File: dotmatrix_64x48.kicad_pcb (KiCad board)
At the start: 2 copper layers, 207 x 120 mm, 372 parts, among them J7 Conn_01x04_Female, P1 CONN_01X06, P2 CONN_01X06, P3 CONN_01X08, P4 CONN_01X08, Q1 Q_NPN_BCE RN5006, Q10 AO3401, Q11 AO3401, Q12 AO3401, Q13 AO3401, Q14 AO3401, Q15 AO3401, Q16 AO3401, Q17 AO3401, Q18 AO3401, Q19 AO3401, Q2 Q_NPN_BEC, Q20 AO3401, Q21 AO3401, Q22 AO3401, Q23 AO3401, Q24 AO3401, Q25 AO3401, Q26 AO3401, Q27 AO3401, Q28 AO3401, Q29 AO3401, Q3 NJL7302L-F3, Q30 Q_NPN_BEC, Q4 Q_NPN_BEC, Q5 AO3401, Q6 AO3401, Q7 AO3401, Q8 AO3401, Q9 AO3401, SW1 SW_PUSH_SMALL_H, SW2 SW_PUSH_SMALL_H, SW3 SW_PUSH_SMALL_H, SW4 SW_PUSH_SMALL_H, SW5 SW_PUSH_SMALL_H, SW6 SW_PUSH_SMALL_H, SW7 SW_PUSH_SMALL_H, SW8 SW_PUSH_SMALL_H, T1 COMMON_MODE_CHOKE, U1 74VHC541, U10 LED1642GW, U11 74HC595, U12 AE-BME280, U13 74HC595, U14 MAX98357, U15 74HC595, U16 ESP32-WROOM, U17 OSRB38C9AA, U18 BME280, U19 TPS54428DDA, U2 TPS54202, U20 CP2102N-A01-GQFN28, U21 CM1293A-04SO, U22 CM1293A-04SO, U23 CM1293A-04SO, U24 CM1293A-04SO, U25 CM1293A-04SO, U3 LED1642GW, U4 LED1642GW, U5 LED1642GW, U6 LED1642GW, U7 LED1642GW, U8 LED1642GW, U9 LED1642GW

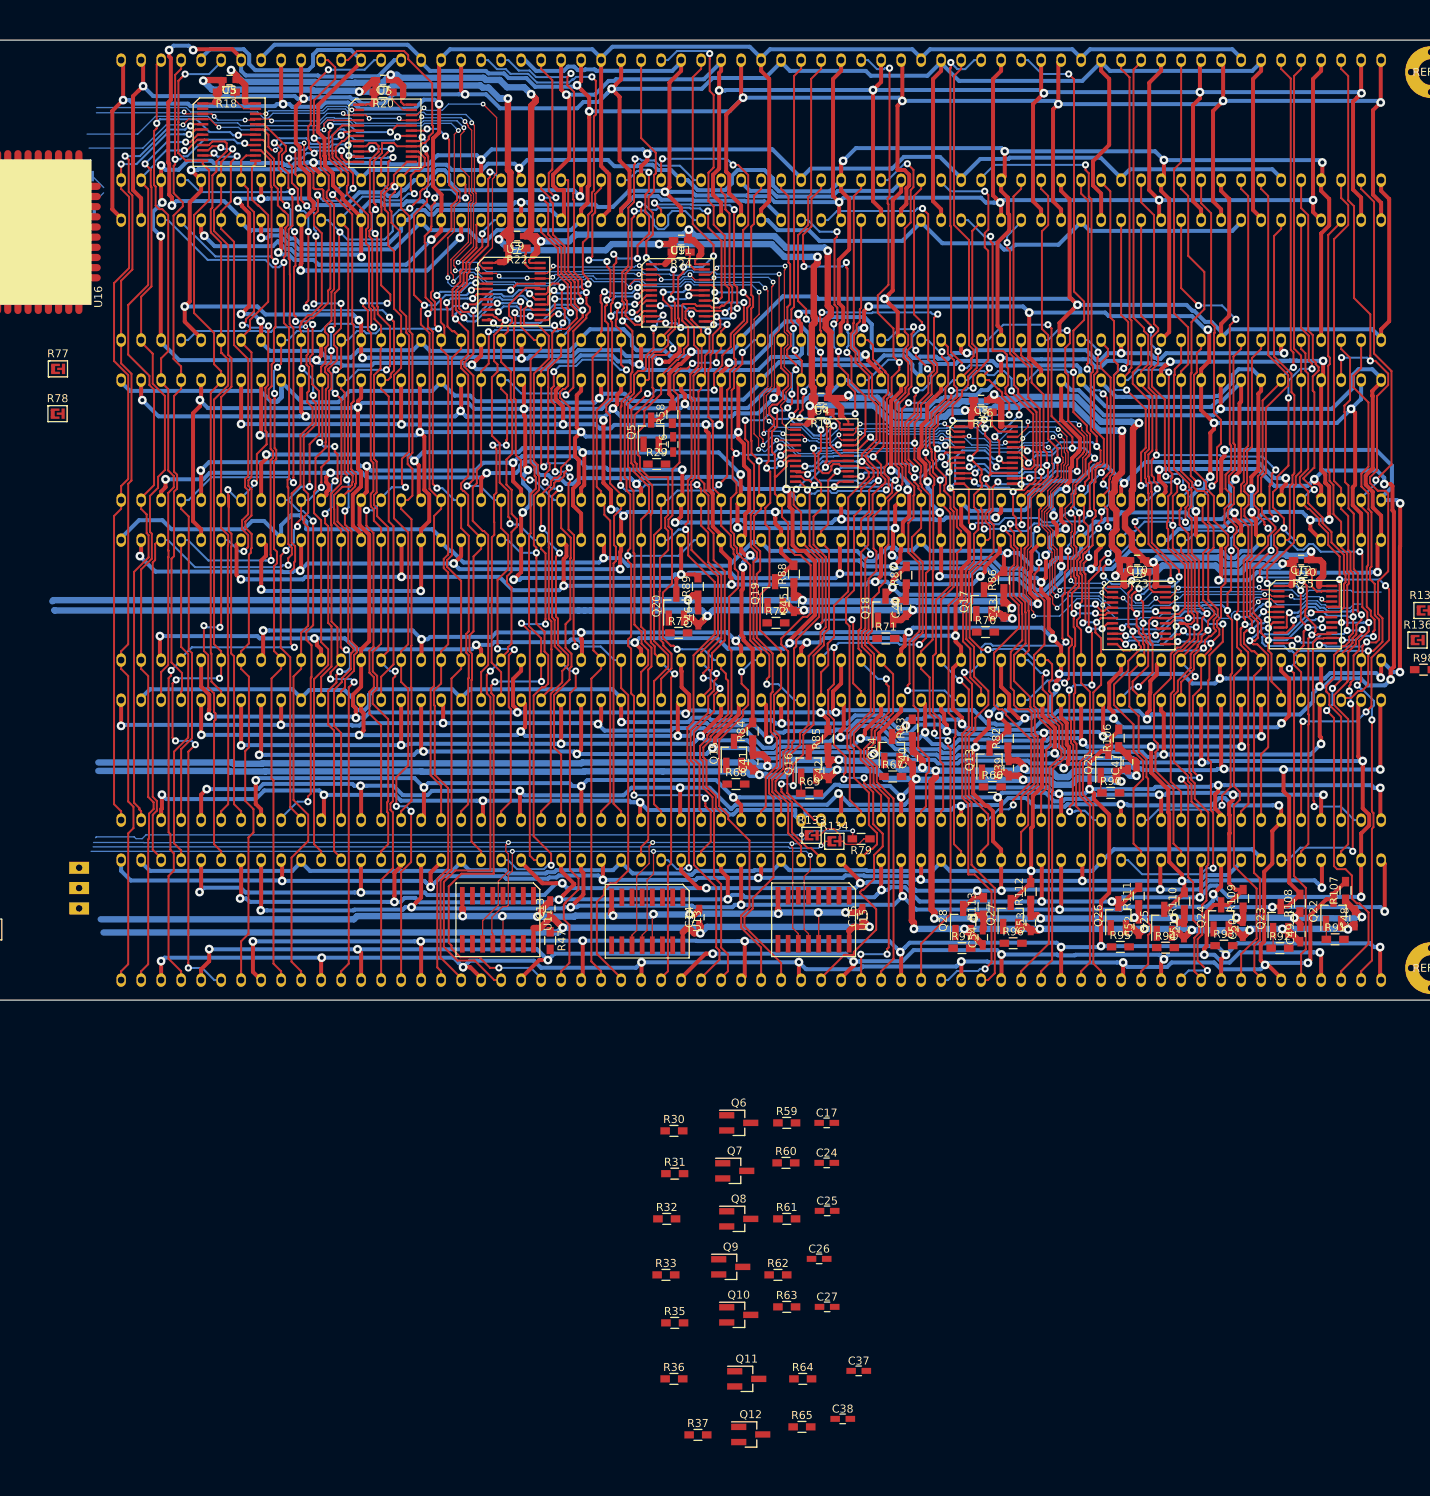
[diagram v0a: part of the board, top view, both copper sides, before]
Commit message: Getting very mojai
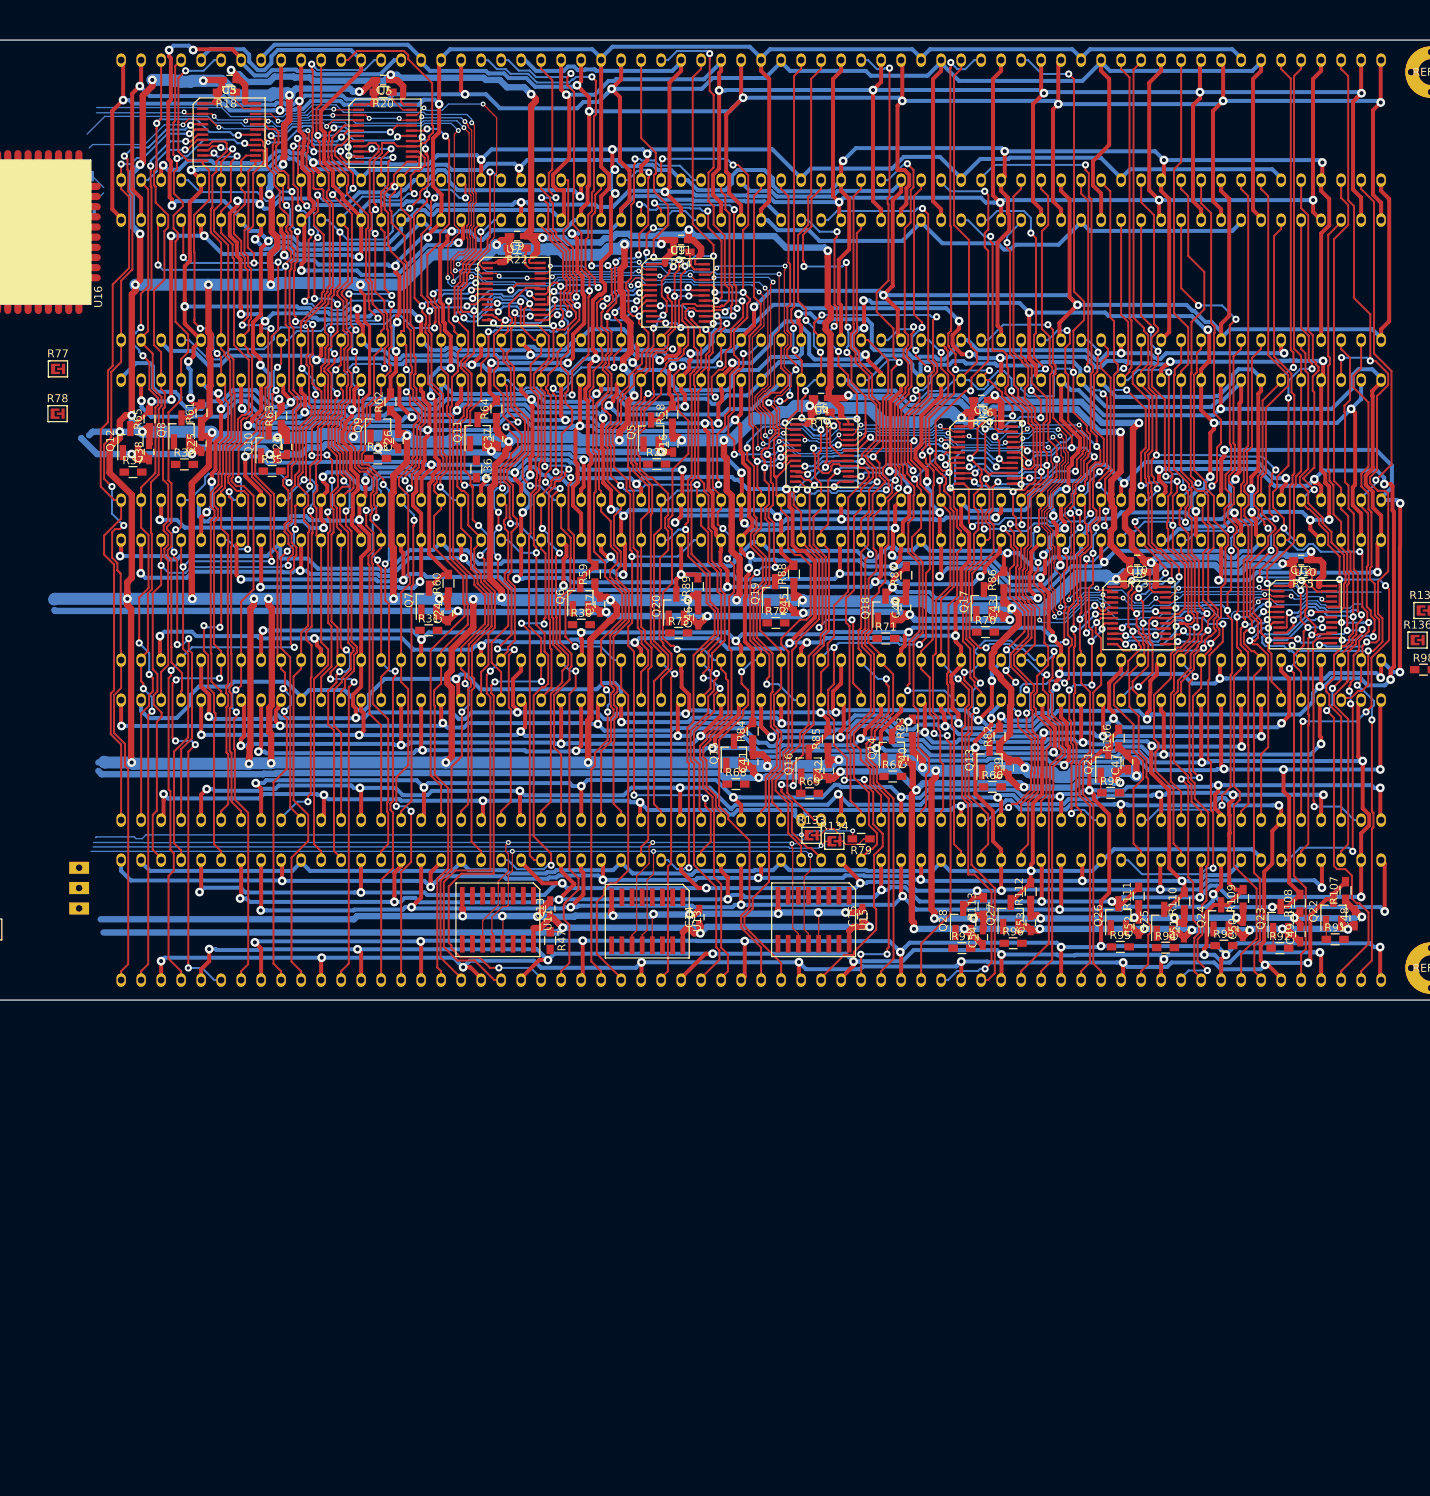
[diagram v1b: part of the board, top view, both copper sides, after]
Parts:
- moved R65 150.1 mm to (121.8, 63.4), turned to 90 degrees
- moved C38 148.7 mm to (121.7, 67.5), turned to 90 degrees
- moved Q12 146.4 mm to (119.4, 66.1), turned to 90 degrees
- moved R37 139.5 mm to (119.7, 70.0)
- moved R63 128.1 mm to (138.3, 63.0), turned to 90 degrees
- moved R64 127.1 mm to (165.2, 62.1), turned to 90 degrees
- moved C27 126.9 mm to (139.0, 66.8), turned to 90 degrees
- moved C37 124.9 mm to (165.4, 65.9), turned to 90 degrees
- moved R61 124.5 mm to (128.3, 62.6), turned to 90 degrees
- moved C25 123.8 mm to (128.3, 66.5), turned to 90 degrees
- moved Q10 123.7 mm to (136.7, 66.5), turned to 90 degrees
- moved Q11 123.1 mm to (162.8, 65.0), turned to 90 degrees
- moved Q8 120.7 mm to (125.8, 64.7), turned to 90 degrees
- moved R62 119.4 mm to (151.9, 61.2), turned to 90 degrees
- moved R35 117.8 mm to (137.1, 69.9)
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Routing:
- net GND: track 829.2 -> 1334.7 mm, vias 38 -> 75
- net LEDVDD: track 531.7 -> 635.3 mm, vias 20 -> 28
- net r2: track 317.5 -> 370.1 mm, vias 8 -> 11
- net r6: track 336.3 -> 380.4 mm, vias 6 -> 9
- net r1: track 354.3 -> 397.1 mm, vias 13 -> 14
- net r15: track 357.0 -> 389.9 mm, vias 15 -> 21
- net r7: track 330.9 -> 361.9 mm, vias 8 -> 11
- net r5: track 336.4 -> 363.9 mm, vias 9 -> 12
- net r4: track 331.7 -> 351.7 mm, vias 5 -> 8
- net r3: track 344.3 -> 359.5 mm, vias 11 -> 12
- net co18: track 94.7 -> 104.9 mm, vias 3 -> 8
- net r12: track 354.1 -> 361.9 mm, vias 5 -> 7
- net r22: track 341.7 -> 349.4 mm, vias 7 -> 8
- net r14: track 363.2 -> 369.7 mm, vias 19 -> 18
- net ce52: track 110.5 -> 116.9 mm, vias 8 -> 10
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
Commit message: Almost all components has placed.
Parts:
- removed C36: 1u, Capacitors_SMD:C_0603_HandSoldering
- removed C63: 0.1u, Capacitors_SMD:C_0603_HandSoldering
- removed P3, P4: CONN_01X08, Pin_Headers:Pin_Header_Straight_1x08_Pitch2.54mm
- removed R1: 1k, Resistors_SMD:R_0603_HandSoldering
- removed U18: BME280, components:BME280-handsoldering
- removed W1, W10, W12, W13, W14, W15, W16, W17, W18, W19, W2, W3, W4, W7: TEST_1P, Measurement_Points:Measurement_Point_Round-SMD-Pad_Small
- added J1: Conn_02x04_Odd_Even, Pin_Headers:Pin_Header_Angled_2x04_Pitch2.54mm, F.Cu at (107.0, 22.2)
- added J2: Conn_02x04_Odd_Even, Pin_Headers:Pin_Header_Angled_2x04_Pitch2.54mm, F.Cu at (114.6, 123.0)
- added REF**: SPK_DAEX25FHE-4_adhesive_circle, components:SPK_DAEX25FHE-4_adhesive_circle, F.Cu at (185.7, 75.9)
- C2, C21, C22, C23, C3, C4, C62, C64, C65, C66, C72, D12, D14, D7, F1, L3, L6, LED49, LED50, LED51, Q1, Q3, R100, R11, R118, R119, R12, R120, R121, R125, R126, R127, R128, R13, R130, R131, R132, R14, R15, R2, R27, R34, R4, R41, R42, R46, R49, R5, R51, R54, R55, R57, R6, R7, R74, R75, R76, R8, U1, U12, U16: moved to B.Cu
- C28, C33: value 10u -> 10u 16V
- C75, C76: value 1u -> 1u 16V
- L1: value 2.2uH -> 10uH; footprint components:Choke_SMD_12x12mm_10.4x10.4mm_compat_h4.5mm_handsoldering -> components:Choke_SMD_7.3x7.3_H3.5_handsoldering
- L2: footprint components:Choke_SMD_12x12mm_10.4x10.4mm_compat_h4.5mm_handsoldering -> components:Choke_SMD_7.3x7.3_H3.5_handsoldering
- LS1: footprint components:SPK_35mm_20mm_RECTANGLE_MOUNT -> Wire_Connections_Bridges:WireConnection_1.50mmDrill
- R80, R81: moved to F.Cu
- moved U25 694.8 mm to (86.2, 46.5)
- moved R34 659.0 mm to (103.2, 18.6), turned to 90 degrees
- moved R118 656.7 mm to (104.5, 20.8), turned to 90 degrees
- moved R127 650.6 mm to (107.2, 17.2)
- moved R121 649.6 mm to (106.8, 28.1), turned to 270 degrees
- moved R119 649.6 mm to (103.0, 28.1), turned to 90 degrees
- moved R120 647.9 mm to (104.2, 28.1), turned to 90 degrees
- moved R128 647.6 mm to (98.0, 53.4), turned to 90 degrees
- moved R132 647.4 mm to (108.8, 53.4), turned to 90 degrees
- moved R130 644.4 mm to (105.8, 53.4), turned to 90 degrees
- moved U22 644.1 mm to (94.7, 104.9), turned to 90 degrees
- moved R126 642.5 mm to (111.1, 17.2)
- moved R122 640.6 mm to (117.1, 21.0), turned to 90 degrees
- moved U21 640.1 mm to (103.0, 132.0), turned to 90 degrees
- moved R125 639.4 mm to (114.9, 17.2), turned to 180 degrees
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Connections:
- net DC_IN renamed DC_IN_P
- net Net-(C72-Pad2) renamed /power/DC_IN_N
- net Net-(CONN3-Pad2) renamed /IR_Sensor/IRLED_K
- net Net-(LS1-Pad1) renamed /IR_Sensor/SPK_P
- net Net-(LS1-Pad2) renamed /IR_Sensor/SPK_N
- C1 pad 1: Net-(C1-Pad1) -> /IR_Sensor/FILT_VDD
- C32 pad 1: Net-(C1-Pad1) -> /IR_Sensor/FILT_VDD
- C4 pad 1: VCC -> LEDVDD
- C67 pad 1: GND -> /USB_UART/USB3V3
- C70 pad 1: GND -> /USB_UART/USB3V3
- C73 pad 1: GND -> /USB_UART/USB3V3
- J7 pad 4: ESPVDD -> LEDLOGICVDD
- L6 pad 1: VCC -> LEDVDD
- P2 pad 1: GND -> /USB_UART/USB3V3
- R10 pad 2: ESPVDD -> LEDLOGICVDD
- R117 pad 2: GND -> /USB_UART/USB3V3
- R123 pad 1: Net-(C1-Pad1) -> /IR_Sensor/FILT_VDD
- R124 pad 1: Net-(C1-Pad1) -> /IR_Sensor/FILT_VDD
- R16 pad 2: VCC -> LEDVDD
- R17 pad 2: VCC -> LEDVDD
- R26 pad 2: VCC -> LEDVDD
- R28 pad 1: ESPVDD -> LEDLOGICVDD
- R45 pad 2: ESPVDD -> /IR_Sensor/FILT_VDD
- R9 pad 2: ESPVDD -> LEDLOGICVDD
- U12 pad 1: ESPVDD -> LEDLOGICVDD
- U17 pad 3: Net-(C1-Pad1) -> /IR_Sensor/FILT_VDD
- U20 pad 6: GND -> /USB_UART/USB3V3
- U21 pad 5: ESPVDD -> LEDLOGICVDD
- U22 pad 5: ESPVDD -> LEDLOGICVDD
- U23 pad 5: ESPVDD -> LEDLOGICVDD
- U24 pad 5: ESPVDD -> LEDLOGICVDD
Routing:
- net GND: track 1334.7 -> 2184.6 mm, vias 75 -> 117
- net /IR_Sensor/IRLED_K: track 0.00 -> 286.9 mm, vias 0 -> 2
- net /CC_GUARD1: track 0.00 -> 272.0 mm, vias 0 -> 8
- net /CC_GUARD0: track 2.03 -> 272.9 mm, vias 0 -> 8
- net Net-(R121-Pad2): track 239.7 -> 0.00 mm, vias 6 -> 0
- net Net-(R119-Pad1): track 237.7 -> 0.00 mm, vias 6 -> 0
- net IR_IN: track 0.00 -> 234.7 mm, vias 0 -> 12
- net /IR_Sensor/FILT_VDD: track 0.00 -> 217.1 mm, vias 0 -> 8
- net E_AIN: track 0.00 -> 213.7 mm, vias 0 -> 11
- net HC595SEROUT: track 0.00 -> 198.7 mm, vias 0 -> 15
- net LEDVDD: track 635.3 -> 797.9 mm, vias 28 -> 36
- net /row_driver/SEL1: track 0.00 -> 160.1 mm, vias 0 -> 6
- net /row_driver/SEL6: track 0.00 -> 146.5 mm, vias 0 -> 8
- net COLSEROUT: track 0.00 -> 142.6 mm, vias 0 -> 4
- net /row_driver/SEL2: track 0.00 -> 132.7 mm, vias 0 -> 6
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- added copper zone on B.Cu, net GND
- added copper zone on B.Cu, net Net-(C72-Pad1)
- added copper zone on F.Cu, net Net-(C72-Pad1)
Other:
- rule pad_to_mask_clearance: 0.2 -> 0.14
- board text removed: "A(5V)"
- board text removed: "DC5V"
- board text removed: "IR RECV"
- board text removed: "K(OC)"
- board text removed: "Ver 4.0 Proto 1"
- board text removed: "WiFi NTP dot-matrix clock"
- board text removed: "https://github.com/w-dee/dotmatrix_64x48"
